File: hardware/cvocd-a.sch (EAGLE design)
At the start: 78 parts, among them IC1 6N138, IC2 LM324D, IC3 MCP4728_QUAD_DAC, IC4 REG1117, IC5 PIC16F1825SO14, IC6 74HC595D, IC7 74HC595D

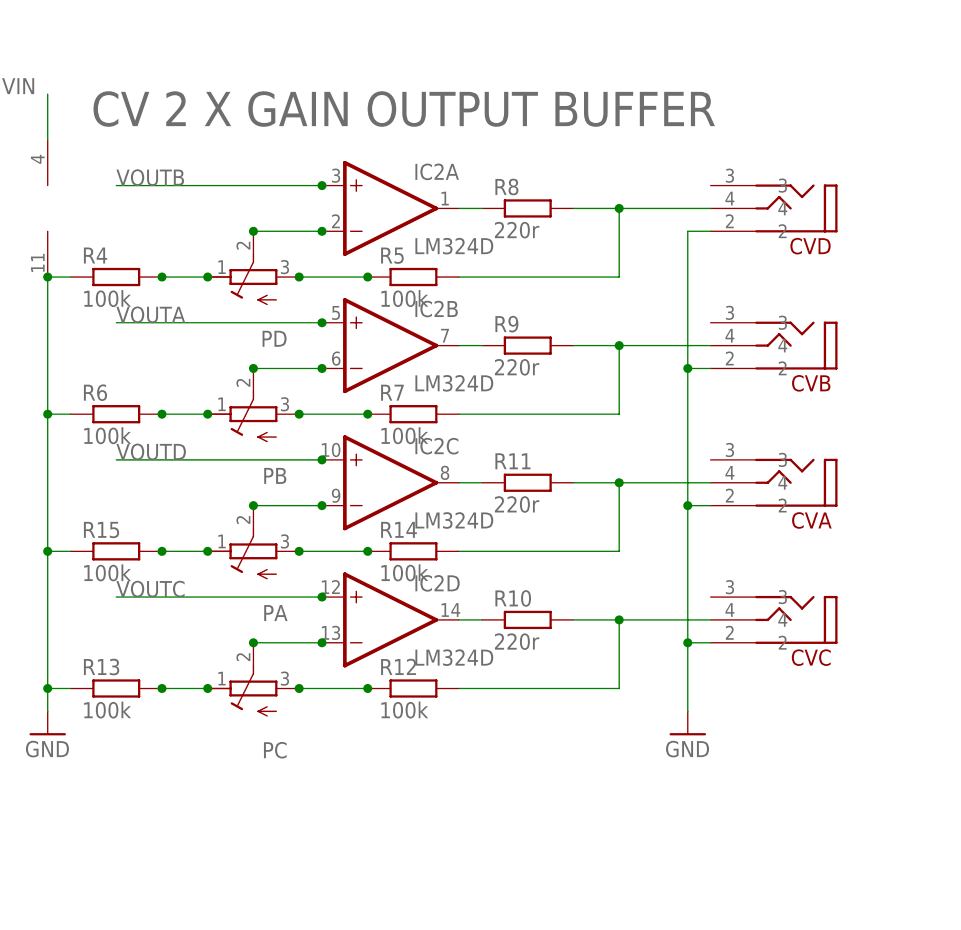
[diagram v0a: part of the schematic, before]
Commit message: v5 board first version
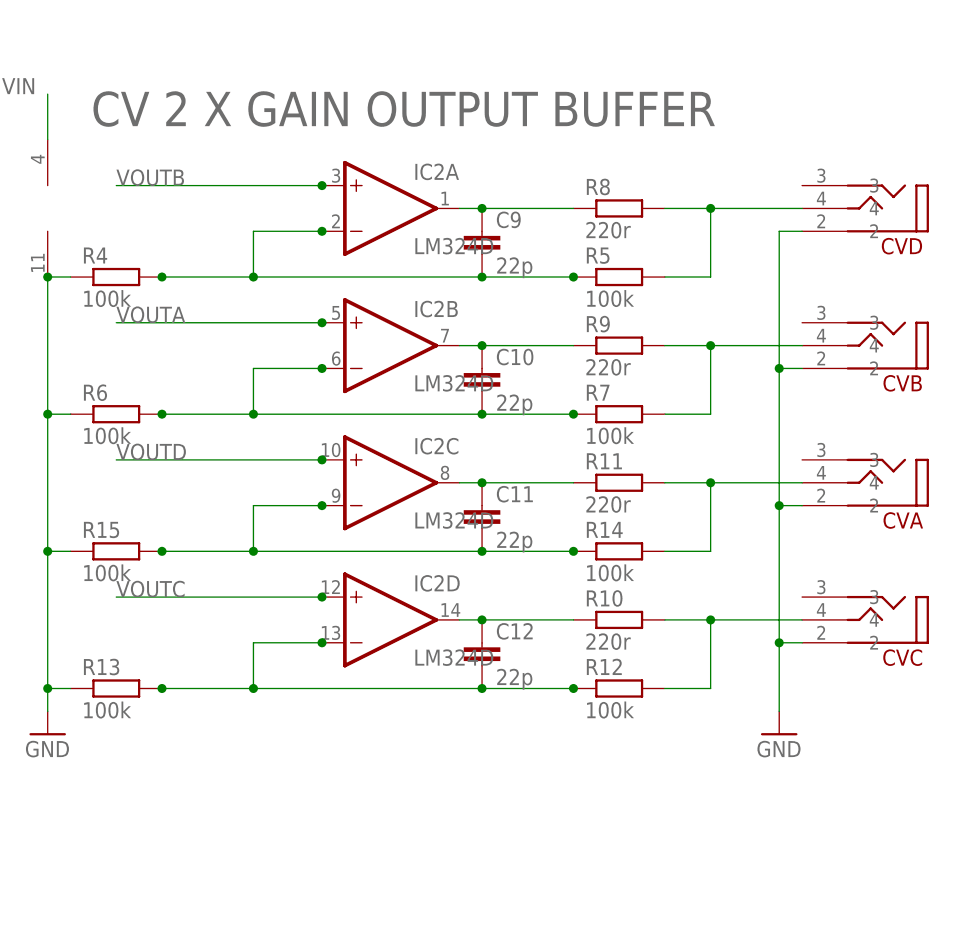
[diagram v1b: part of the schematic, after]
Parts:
- removed PA, PB, PC, PD: (no value), rcl:R-TRIMM3314G
- added C10, C11, C12, C9: 22p, rcl:C-EUC0805
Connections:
- removed net N$17: PD.E, R4.2
- removed net N$25: PD.A, R5.1
- removed net N$27: PB.E, R6.2
- removed net N$28: PB.A, R7.1
- removed net N$45: PA.E, R15.2
- removed net N$54: PA.A, R14.1
- removed net N$55: PC.E, R13.2
- removed net N$56: PC.A, R12.1
- net N$10: now also C9.2, R4.2, R5.1; no longer PD.S
- net N$11: now also C11.2, R14.1, R15.2; no longer PA.S
- net N$14: now also C12.2, R12.1, R13.2; no longer PC.S
- net N$2: now also C9.1
- net N$26: now also C10.2, R6.2, R7.1; no longer PB.S
- net N$3: now also C10.1
- net N$4: now also C11.1
- net N$5: now also C12.1
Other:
- moved on the sheet: CVA, CVB, CVC, CVD, R10, R11, R12, R14, R5, R7, R8, R9
